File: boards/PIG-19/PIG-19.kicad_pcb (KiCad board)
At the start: 2 copper layers, 70 x 40 mm, 43 parts, among them J1 XT30PW-F, J11 USB4105-GF-A, J2 XT30PW-F, J5 Conn_01x02_Pin, J6 Conn_01x02_Pin, J9 XT30PW-M, Q1 PMOS, SW3 SW_Nidec_CAS-120A1, U1 LM2940S-5.0

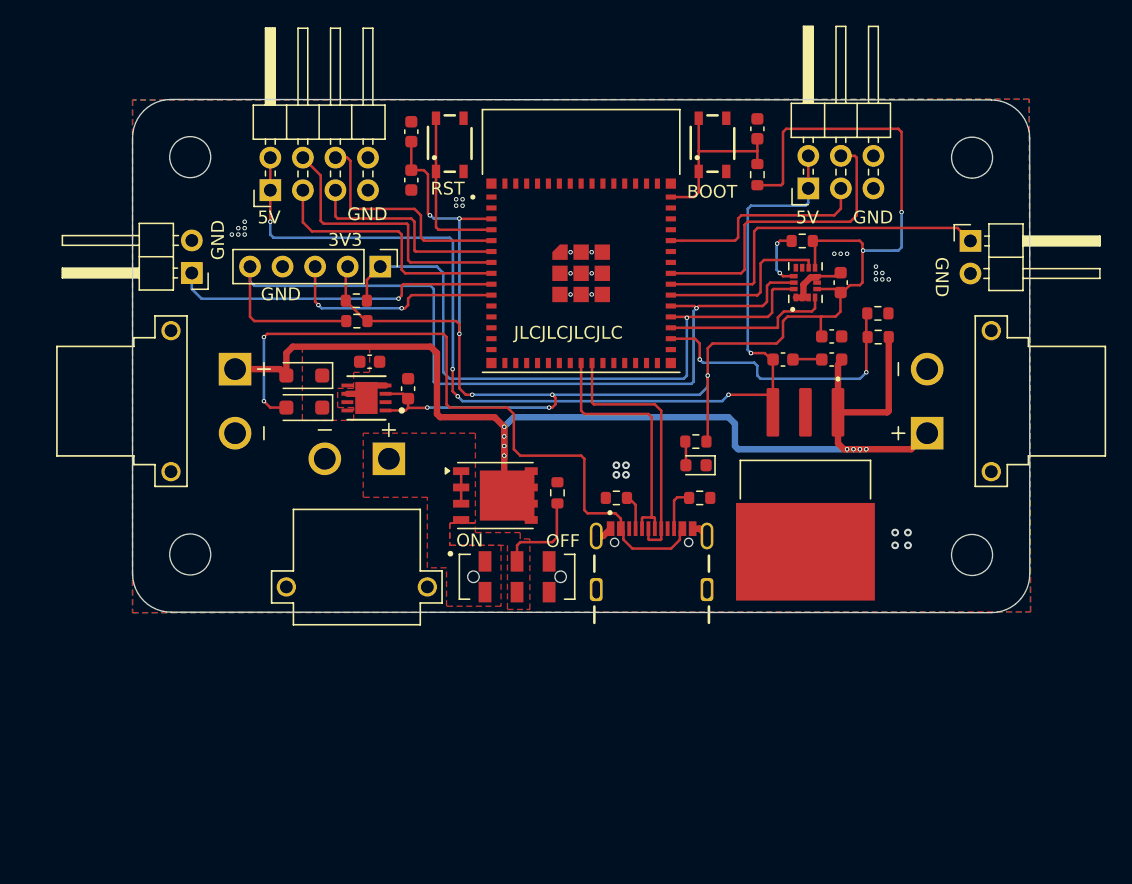
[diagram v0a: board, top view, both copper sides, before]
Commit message: board updates
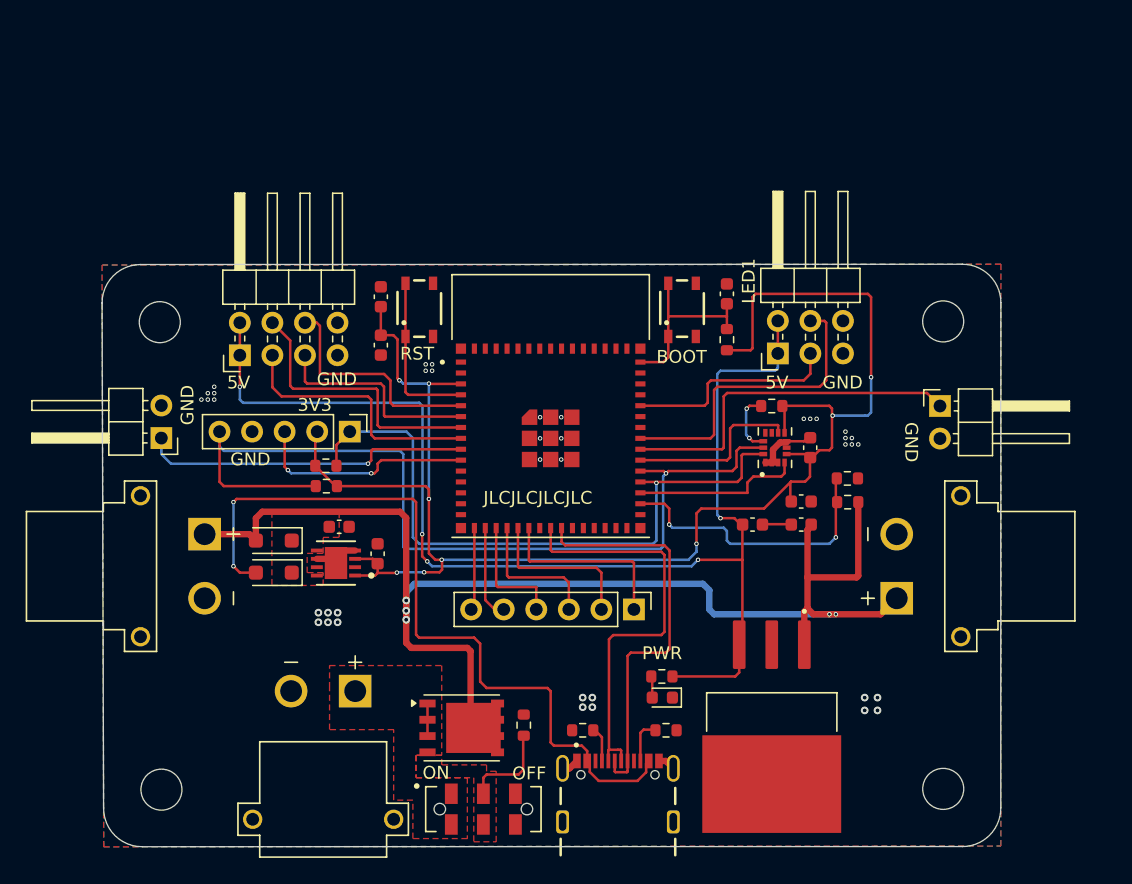
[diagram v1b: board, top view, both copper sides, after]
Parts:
- added RescueDCPin1: Conn_01x06_Pin, Connector_PinHeader_2.54mm:PinHeader_1x06_P2.54mm_Vertical, F.Cu at (166.4, 81.5)
- R1: value 510 -> 100
- R8: value 470k -> 1M
- R9: value 530k -> 500k
- moved R1 18.5 mm to (168.5, 86.7)
- moved H2 18.5 mm to (129.5, 95.6)
- moved H3 18.4 mm to (190.5, 95.5)
- moved Q1 18.3 mm to (152.9, 90.7)
- moved J9 18.3 mm to (142.1, 97.9)
- moved R5 18.3 mm to (168.9, 90.9)
- moved R6 18.3 mm to (162.4, 90.9)
- moved U1 18.3 mm to (177.1, 90.6)
- moved D1 18.3 mm to (168.6, 88.4)
- moved R2 18.3 mm to (157.8, 90.5)
- moved J11 18.3 mm to (165.1, 98.1)
- moved SW3 18.3 mm to (154.6, 97.1)
- moved R10 13.1 mm to (142.3, 70.3)
- moved R9 13.1 mm to (183.0, 71.3)
- moved C3 13.1 mm to (173.6, 56.9)
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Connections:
- MCU1 pad 16: unconnected-(MCU1-IO12-Pad16) -> /ENB
- MCU1 pad 17: unconnected-(MCU1-IO13-Pad17) -> /IN4
- MCU1 pad 18: unconnected-(MCU1-IO14-Pad18) -> /IN3
- MCU1 pad 19: unconnected-(MCU1-IO15-Pad19) -> /IN2
- MCU1 pad 20: unconnected-(MCU1-IO16-Pad20) -> /IN1
- MCU1 pad 21: unconnected-(MCU1-IO17-Pad21) -> /ENA
- R1 pad 1: +3V3 -> +5V
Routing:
- net /ENA: track 0.00 -> 14.4 mm
- net /DN: track 19.9 -> 32.6 mm
- net /IN1: track 0.00 -> 12.6 mm
- net +3V3: track 138.8 -> 126.3 mm, vias 10 -> 9
- net +BATT: track 95.9 -> 108.1 mm, vias 8 -> 5
- net +5V: track 85.0 -> 96.5 mm
- net /DP: track 20.6 -> 31.9 mm
- net /IN2: track 0.00 -> 10.9 mm
- net /IN3: track 0.00 -> 9.40 mm
- net /IN4: track 0.00 -> 7.36 mm
- net /ENB: track 0.00 -> 6.45 mm
- net +V_USB: track 55.6 -> 60.6 mm
- net GND: vias 33 -> 39
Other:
- board size 70 x 40 mm -> 70.1 x 45.4 mm
- board text added: "PWR"
